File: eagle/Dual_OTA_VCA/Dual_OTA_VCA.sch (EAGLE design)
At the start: 37 parts, among them IC1 LM13600N, IC2 NJM4580, IC3 LM4558N, T1 2SA1015

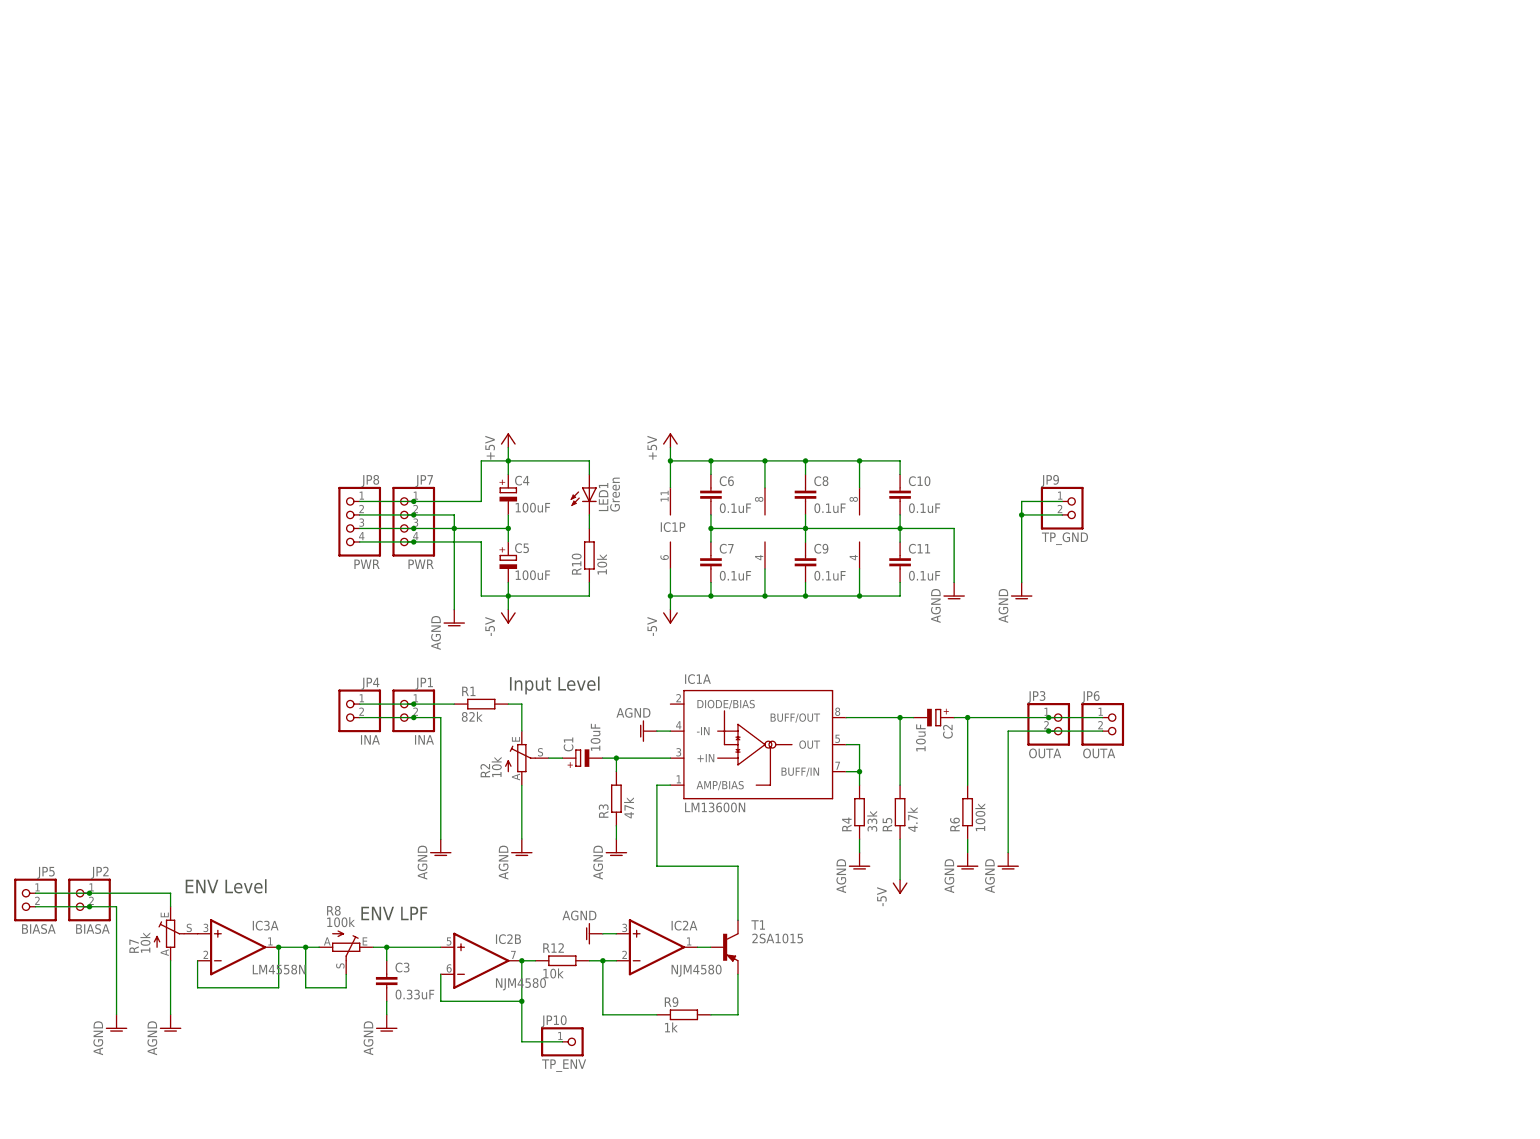
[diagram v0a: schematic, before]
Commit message: begin 2ch
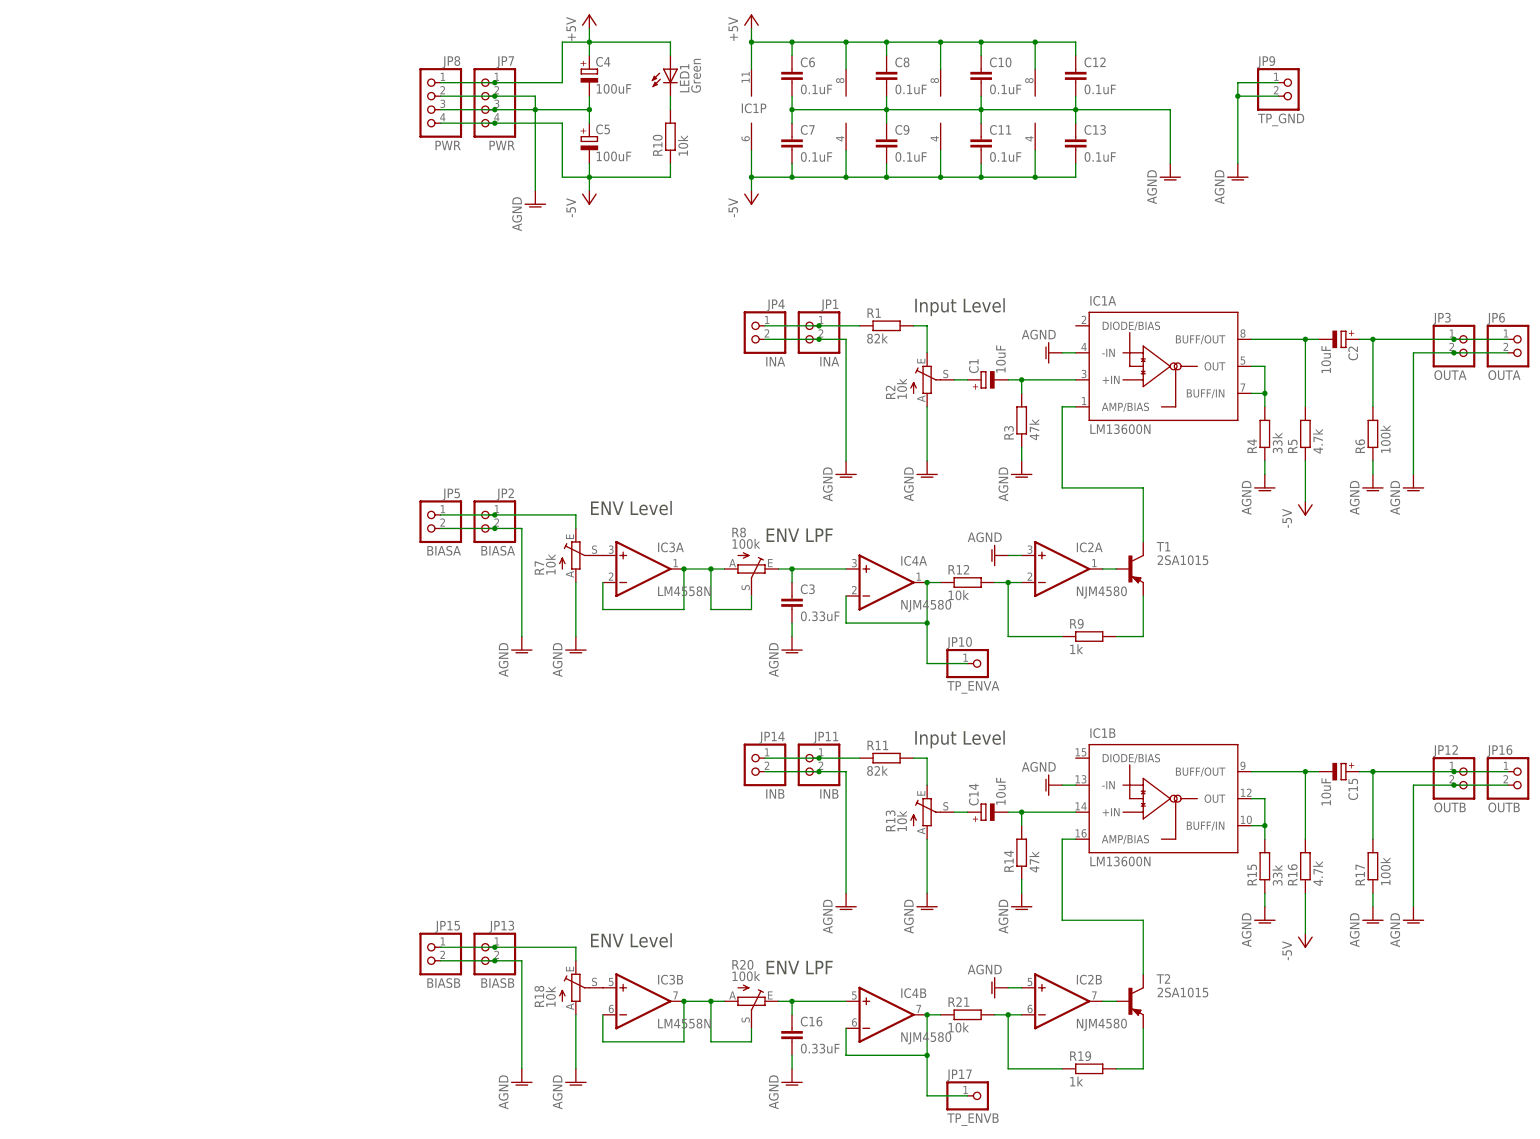
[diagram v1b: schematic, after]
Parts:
- added C12, C13: 0.1uF, rcl:C-EU025-024X044
- added C14, C15: 10uF, rcl:CPOL-EUE2.5-7
- added C16: 0.33uF, rcl:C-EU050-030X075
- added IC4: NJM4580, linear:LM4558N
- added JP11, JP14: INB, pinhead:PINHD-1X2
- added JP12, JP16: OUTB, pinhead:PINHD-1X2
- added JP13, JP15: BIASB, pinhead:PINHD-1X2
- added JP17: TP_ENVB, pinhead:PINHD-1X1
- added R11: 82k, rcl:R-EU_0207/7
- added R13, R18: 10k, pot:TRIM_EU-B25P
- added R14: 47k, rcl:R-EU_0207/7
- added R15: 33k, rcl:R-EU_0207/7
- added R16: 4.7k, rcl:R-EU_0207/7
- added R17: 100k, rcl:R-EU_0207/7
- added R19: 1k, rcl:R-EU_0207/7
- added R20: 100k, pot:TRIM_EU-B25P
- added R21: 10k, rcl:R-EU_0207/7
- added T2: 2SA1015, transistor-neu-to92:-PNP-TO92-ECB
- JP10: value TP_ENV -> TP_ENVA
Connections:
- new net N$13: IC3B.+IN, R18.S
- new net N$16: JP11.1, JP14.1, R11.1
- new net N$20: R11.2, R13.E
- new net N$21: C14.+, R13.S
- new net N$22: C14.-, IC1B.+IN, R14.2
- new net N$23: IC1B.BUFF/IN, IC1B.OUT, R15.2
- new net N$24: C15.-, IC1B.BUFF/OUT, R16.2
- new net N$25: C15.+, JP12.1, JP16.1, R17.2
- new net N$26: JP13.1, JP15.1, R18.E
- new net N$27: IC2B.-IN, R19.1, R21.2
- new net N$28: R19.2, T2.E
- new net N$29: IC2B.OUT, T2.B
- new net N$30: IC1B.AMP/BIAS, T2.C
- new net N$32: IC3B.-IN, IC3B.OUT, R20.A, R20.S
- new net N$33: C16.1, IC4B.+IN, R20.E
- new net N$34: IC4B.-IN, IC4B.OUT, JP17.1, R21.1
- net +5V: now also C12.1, IC4P.V+
- net -5V: now also C13.2, IC4P.V-, R16.1
- net AGND: now also C12.2, C13.1, C16.2, IC1B.-IN, IC2B.+IN, JP11.2, JP12.2, JP13.2, JP14.2, JP15.2, JP16.2, R13.A, R14.1, R15.1, R17.1, R18.A
- net N$19: now also IC4A.+IN; no longer IC2B.+IN
- net N$7: now also IC4A.-IN, IC4A.OUT; no longer IC2B.-IN, IC2B.OUT
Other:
- moved on the sheet: C1, C10, C11, C2, C3, C4, C5, C6, C7, C8, C9, IC1A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

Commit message: Update the eagle files
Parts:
- C6, C7: device rcl:C-EU025-024X044 -> rcl:C-EU050-024X044
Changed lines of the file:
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@@
 <part name="LED1" library="led" deviceset="LED" device="3MM" value="Green"/>
 <part name="R10" library="rcl" deviceset="R-EU_" device="0207/7" value="10k"/>
-<part name="C6" library="rcl" deviceset="C-EU" device="025-024X044" value="0.1uF"/>
-<part name="C7" library="rcl" deviceset="C-EU" device="025-024X044" value="0.1uF"/>
+<part name="C6" library="rcl" deviceset="C-EU" device="050-024X044" value="0.1uF"/>
+<part name="C7" library="rcl" deviceset="C-EU" device="050-024X044" value="0.1uF"/>
 <part name="C8" library="rcl" deviceset="C-EU" device="025-024X044" value="0.1uF"/>
 <part name="C9" library="rcl" deviceset="C-EU" device="025-024X044" value="0.1uF"/>
